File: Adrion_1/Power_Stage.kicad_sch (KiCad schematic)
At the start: 85 parts, among them IC4 CKSR_15-NP, J1 Screw_Terminal_01x02, J3 Conn_01x04, Q1 IPT034N15NM6ATMA1, Q2 IPT034N15NM6ATMA1, Q3 IPT034N15NM6ATMA1, Q5 IPT034N15NM6ATMA1, U1 UCC21521DW, U3 UCC21521DW

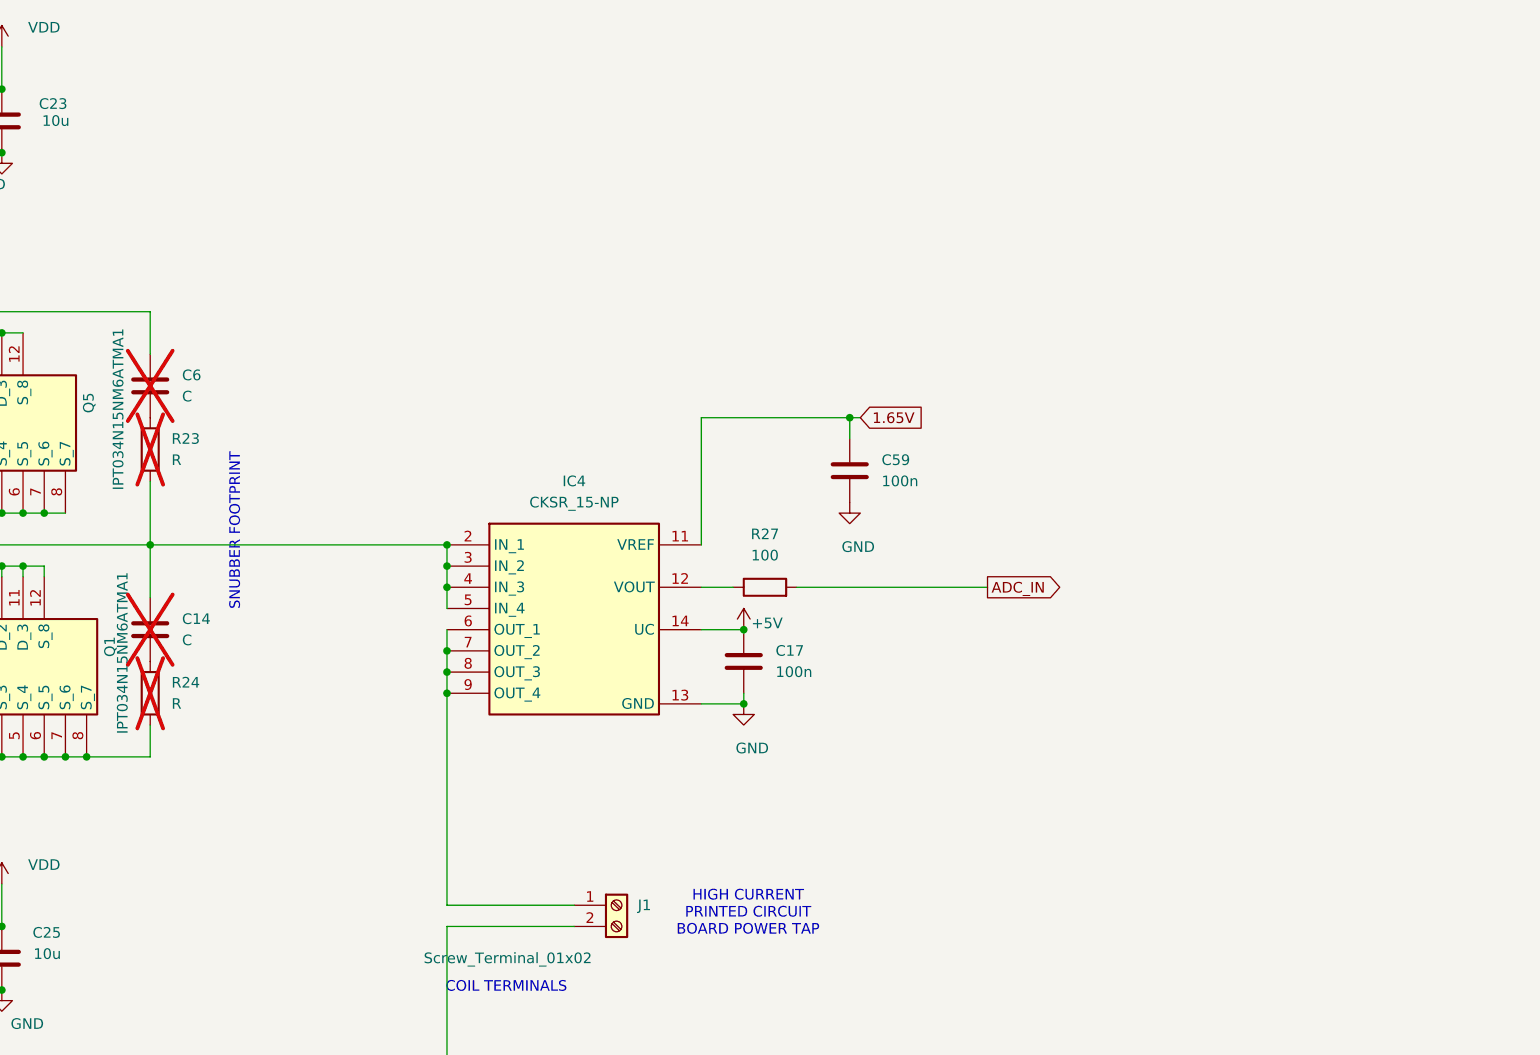
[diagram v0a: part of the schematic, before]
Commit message: Correcciones
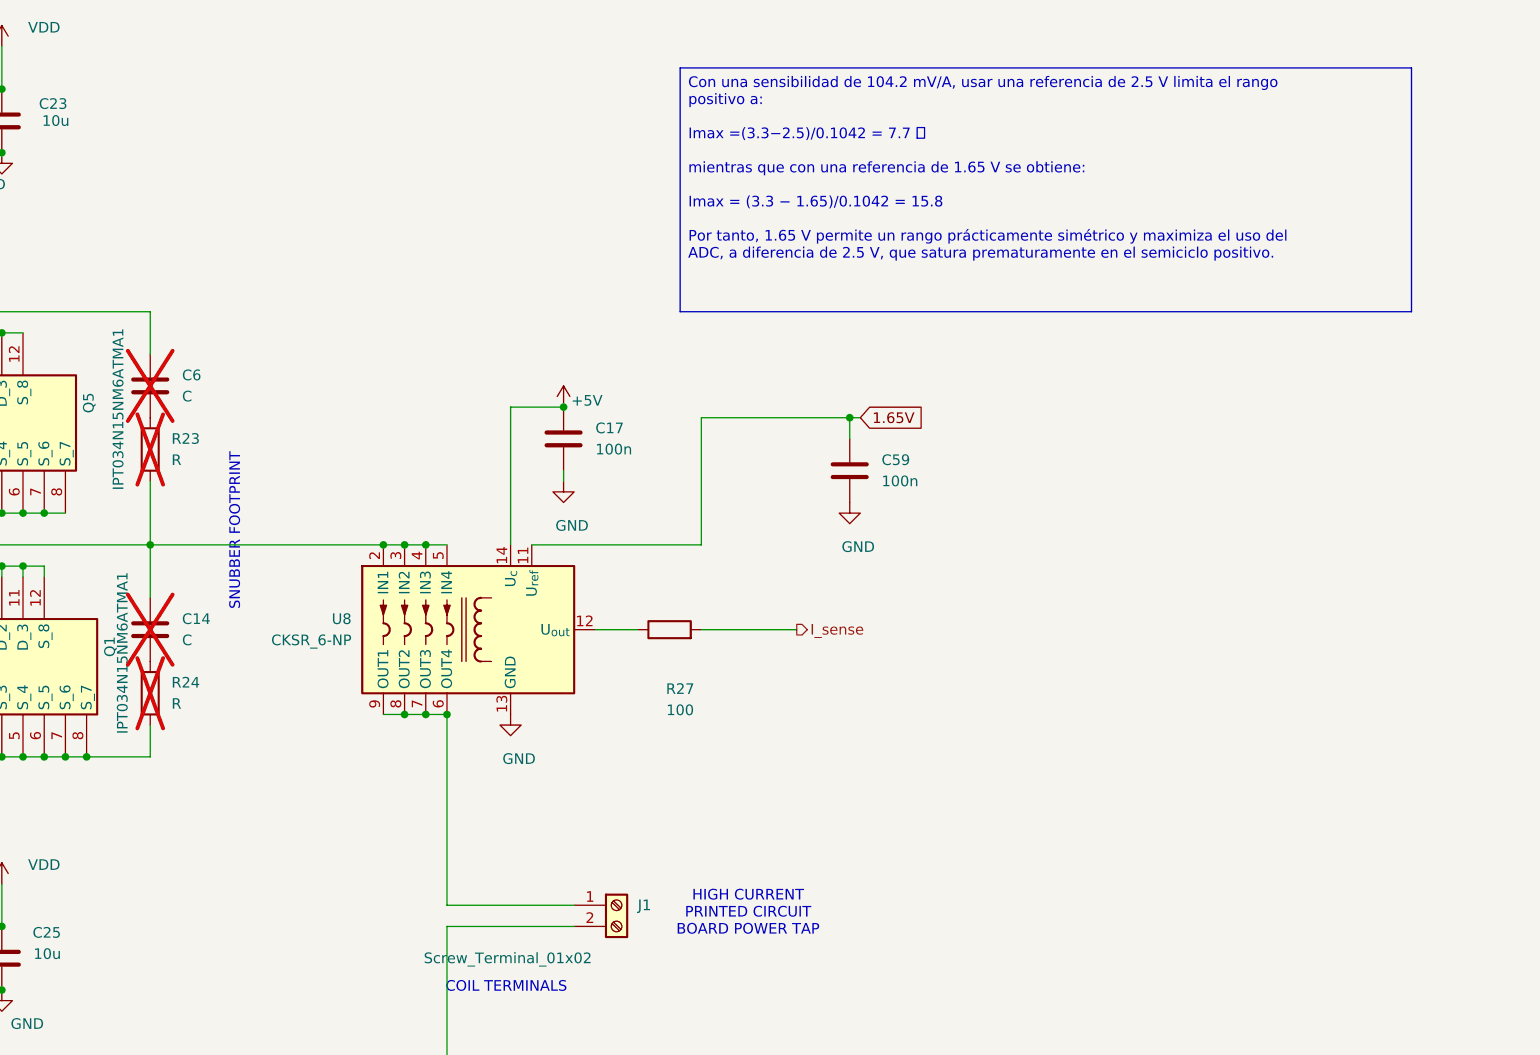
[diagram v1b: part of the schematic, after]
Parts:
- removed IC4: CKSR_15-NP, CKSR15NP, symbol CKSR_15-NP:CKSR_15-NP
- added U8: CKSR_6-NP, Sensor_Current:LEM_CKSR, symbol Sensor_Current:CKSR_6-NP
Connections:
- net +5V: now also U8.14 (U_{c})
- net 1.65V: now also U8.11 (U_{ref})
- net GND: now also U8.13 (GND)
- net at C14.1, C18.2, C19.2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: now also U8.2 (IN1), U8.3 (IN2), U8.4 (IN3), U8.5 (IN4)
- net at R27.1: now also U8.12 (U_{out})
- net at J1.1 (Pin_1): now also U8.6 (OUT4), U8.7 (OUT3), U8.8 (OUT2), U8.9 (OUT1)
- net ADC_IN renamed I_sense
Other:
- moved on the sheet: C17, R27
